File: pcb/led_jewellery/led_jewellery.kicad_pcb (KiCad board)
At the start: 2 copper layers, 12.3 x 25.6 mm, 6 parts, among them J1 Conn_01x01, J2 Conn_01x01, SW1 SW_SPST

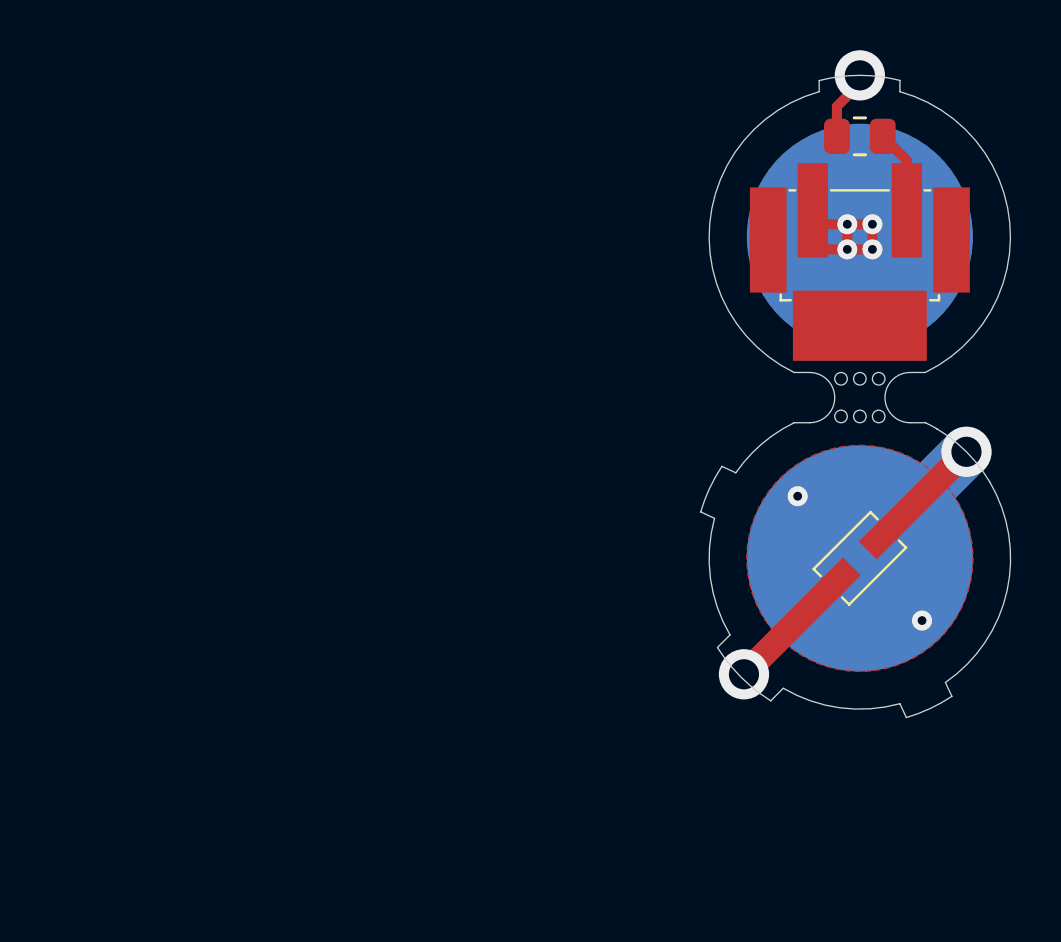
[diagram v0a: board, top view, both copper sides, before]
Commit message: first attempt at PCBA layout, x2 boards
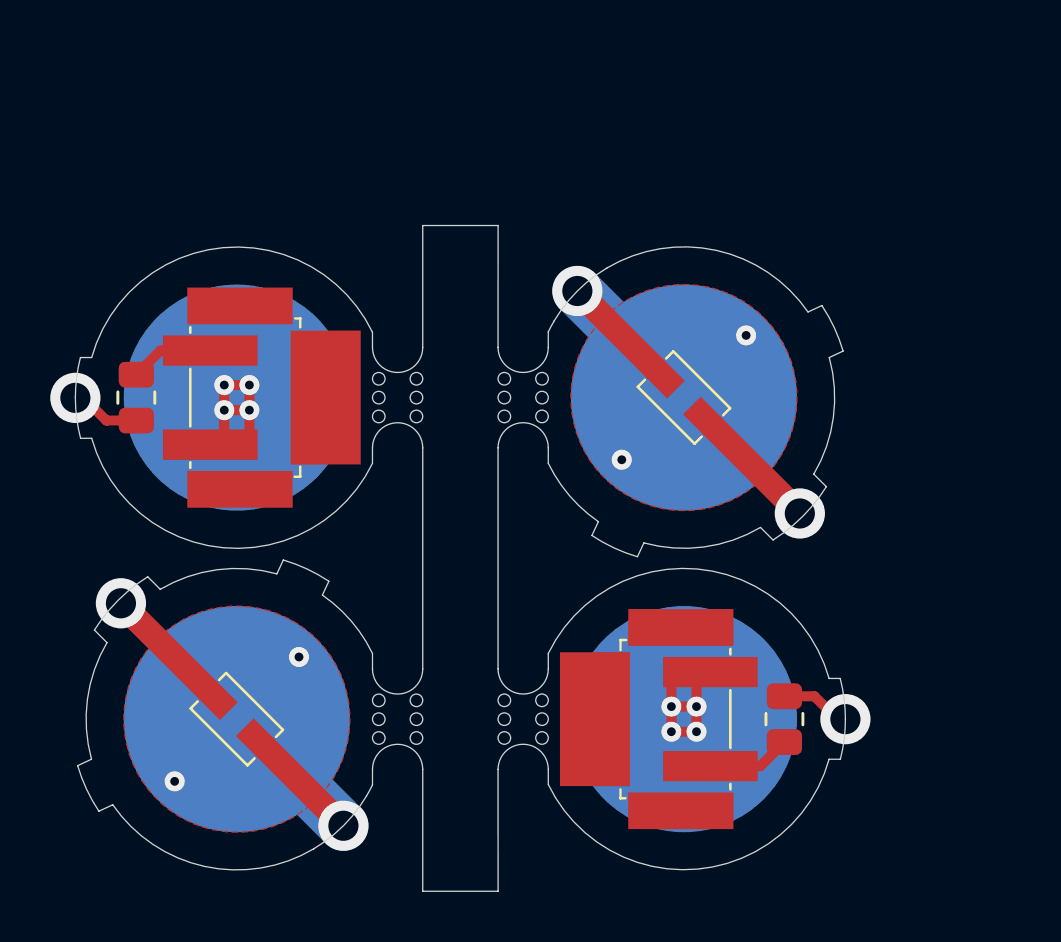
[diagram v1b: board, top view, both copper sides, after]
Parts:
- added D1: LED, led_jewellery:LED, F.Cu at (117.5, 78.4)
- added J1: Conn_01x01, led_jewellery:9mm_pad, B.Cu at (117.5, 78.4)
- added J2: Conn_01x01, led_jewellery:9mm_pad, B.Cu at (117.5, 91.2)
- added R2: R, Resistor_SMD:R_0805_2012Metric, F.Cu at (121.5, 91.2)
- added SW2: SW_SPST, diptronics_ta3:diptronics_ta3, F.Cu at (115.0, 91.2)
- added mouse-bite-2mm-slot: VAL**, mousebites:mouse-bite-2mm-slot, F.Cu at (111.1, 78.4)
- added mouse-bite-2mm-slot: VAL**, mousebites:mouse-bite-2mm-slot, F.Cu at (111.1, 91.2)
- added mouse-bite-2mm-slot: VAL**, mousebites:mouse-bite-2mm-slot, F.Cu at (106.1, 91.2)
- moved R1 30.6 mm to (95.7, 78.4), turned to -90 degrees
- moved J2 25.6 mm to (99.7, 78.4), turned to -90 degrees
- moved D1 25.6 mm to (99.7, 91.2), turned to 135 degrees
- moved J1 25.6 mm to (99.7, 91.2), turned to 135 degrees
- moved SW1 22.6 mm to (102.2, 78.4), turned to 90 degrees
- moved mouse-bite-2mm-slot 18.4 mm to (106.1, 78.4), turned to 90 degrees
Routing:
- net /BAT+: track 9.06 -> 18.1 mm, vias 4 -> 8
- net /BAT-: track 6.00 -> 12.0 mm, vias 3 -> 6
- net /LED+: track 5.30 -> 10.6 mm, vias 2 -> 4
- net Net-(SW1-B): track 3.34 -> 6.69 mm
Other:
- board size 12.3 x 25.6 mm -> 30.7 x 26.5 mm
